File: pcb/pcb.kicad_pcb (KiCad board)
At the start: 2 copper layers, 34 parts, among them J1 Conn_02x08_Odd_Even, J2 B2B-PH-K-S_LF__SN_, J3 USB_C_Receptacle, Q1 MMUN2211LT1G, SW1 SW_SPST, U1 TPS61090, U2 MCP73871-1AA

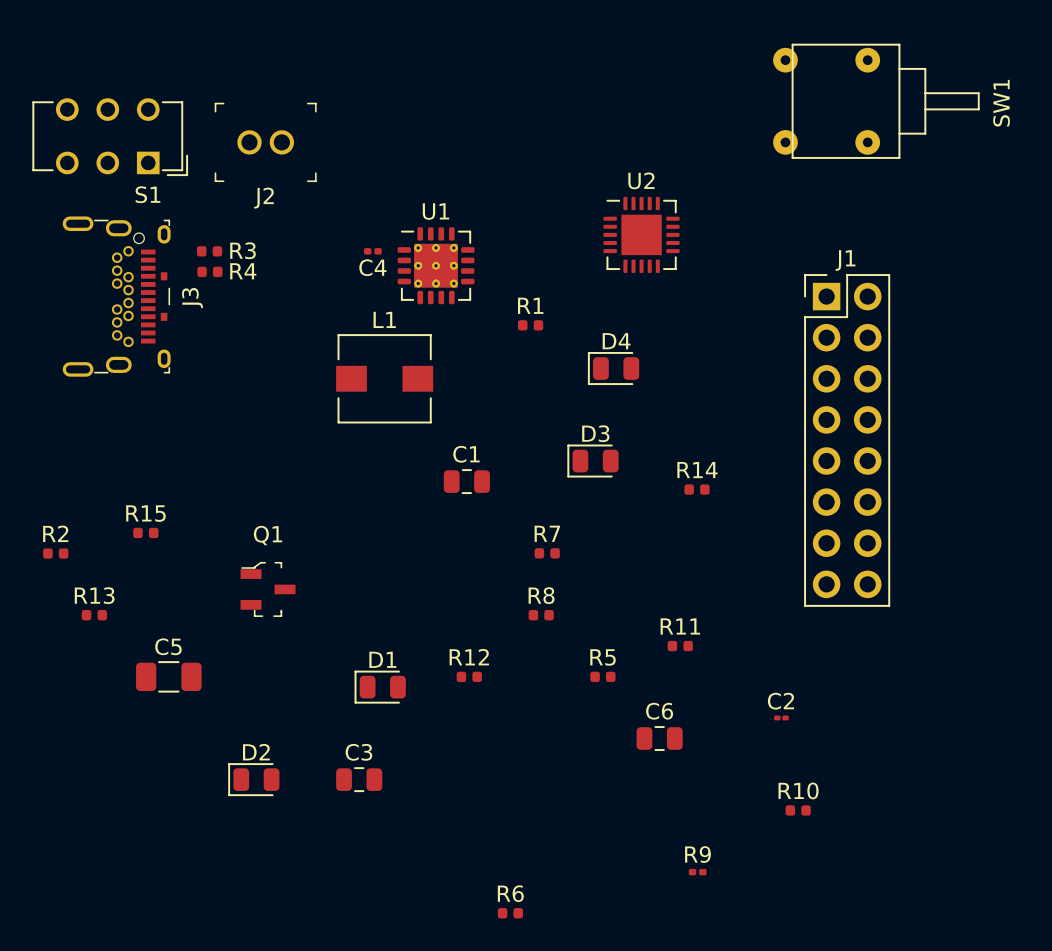
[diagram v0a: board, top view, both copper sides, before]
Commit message: rough positioning of components
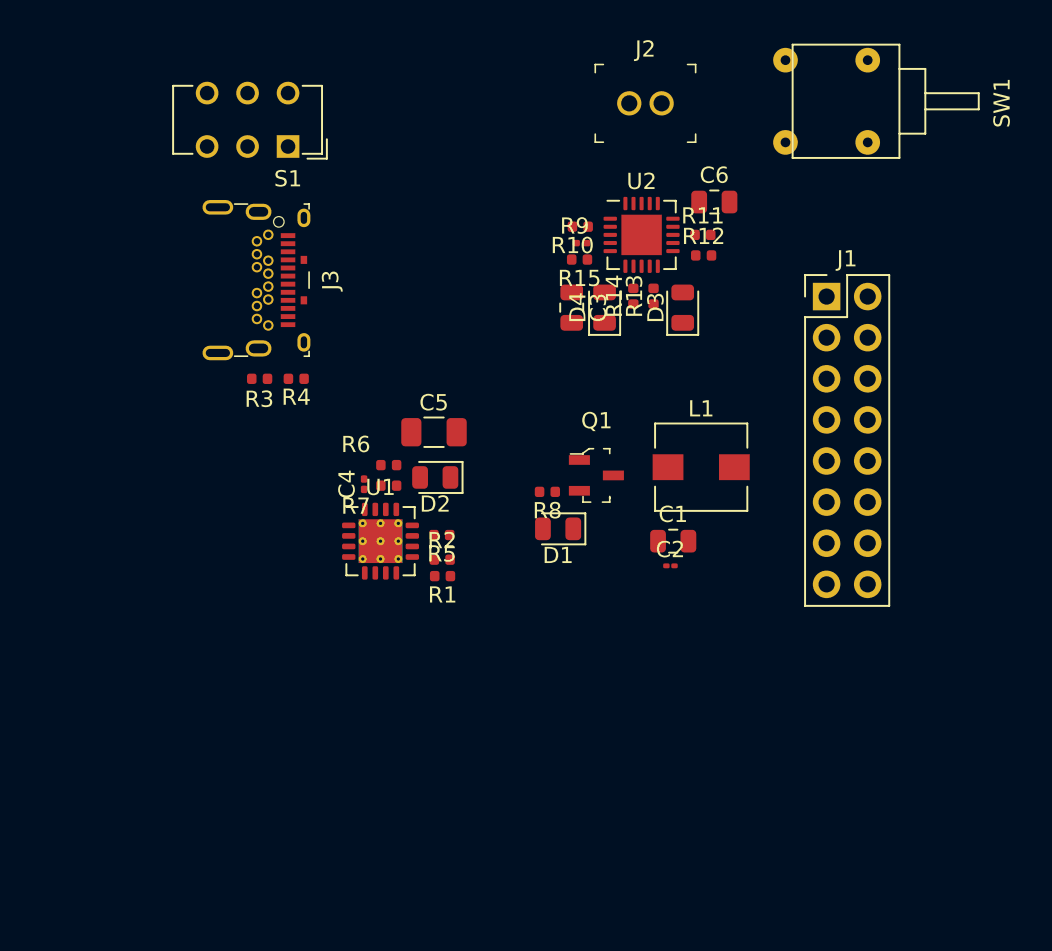
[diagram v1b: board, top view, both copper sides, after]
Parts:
- moved R13 39.8 mm to (201.4, 95.2), turned to 90 degrees
- moved R9 39.5 mm to (196.9, 91.9)
- moved R10 38.5 mm to (196.9, 90.9), turned to 180 degrees
- moved C6 33.3 mm to (205.2, 89.4)
- moved C3 32.0 mm to (196.3, 95.9), turned to 270 degrees
- moved R15 31.7 mm to (196.8, 93.0), turned to 180 degrees
- moved R12 29.8 mm to (204.5, 92.7)
- moved R6 28.7 mm to (185.0, 105.7), turned to 180 degrees
- moved R11 25.4 mm to (204.4, 91.4)
- moved R2 23.9 mm to (188.3, 111.5)
- moved C5 22.3 mm to (187.8, 103.6)
- moved D2 21.7 mm to (187.9, 106.4), turned to 180 degrees
- moved J2 21.6 mm to (199.9, 83.3), turned to 0 degrees
- moved Q1 21.5 mm to (197.9, 106.3)
- moved L1 20.3 mm to (204.3, 105.8)
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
